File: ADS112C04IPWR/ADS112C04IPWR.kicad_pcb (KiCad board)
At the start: 2 copper layers, 22.9 x 22.9 mm, 3 parts, among them J1 Conn_01x08, J2 Conn_01x08, U1 ADS112C04IPWR

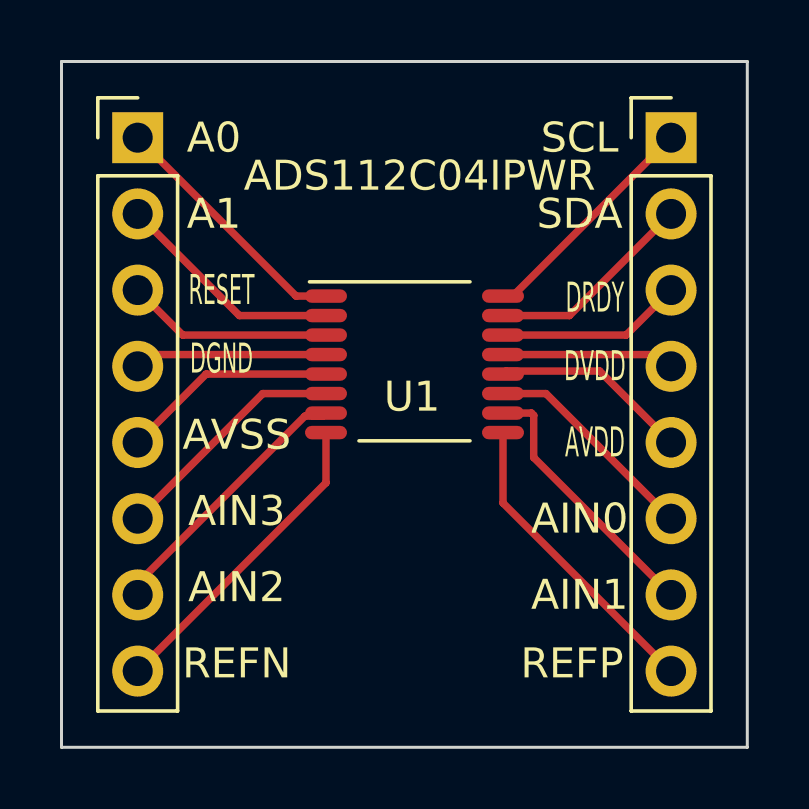
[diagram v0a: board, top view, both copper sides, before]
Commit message: Revision One
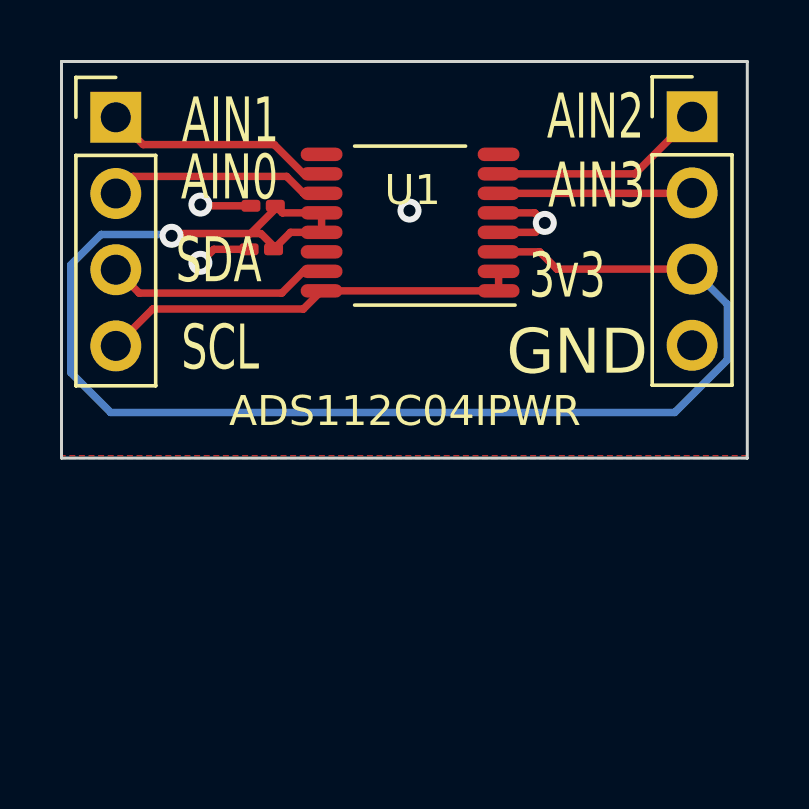
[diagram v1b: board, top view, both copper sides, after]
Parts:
- added C1: 0.1μF, Capacitor_SMD:C_0201_0603Metric_Pad0.64x0.40mm_HandSolder, F.Cu at (149.0, 68.3)
- added C2: 0.1μF, Capacitor_SMD:C_0201_0603Metric_Pad0.64x0.40mm_HandSolder, F.Cu at (148.9, 69.8)
- J1, J2: value Conn_01x08 -> Conn_01x04; footprint Connector_PinHeader_2.54mm:PinHeader_1x08_P2.54mm_Vertical -> Connector_PinHeader_2.54mm:PinHeader_1x04_P2.54mm_Vertical
- moved U1 4.73 mm to (153.9, 68.9), turned to 180 degrees
- moved J1 1.00 mm to (144.1, 65.4)
- moved J2 0.99 mm to (163.3, 65.3)
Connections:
- J1 pad 1: Net-(J1-Pad1) -> /AIN1
- J1 pad 2: Net-(J1-Pad2) -> /AIN0
- J1 pad 3: Net-(J1-Pad3) -> /SDA
- J1 pad 4: GNDD -> /SCL
- J2 pad 1: Net-(J2-Pad1) -> /AIN2
- J2 pad 2: Net-(J2-Pad2) -> /AIN3
- J2 pad 3: Net-(J2-Pad3) -> +3V3
- J2 pad 4: Net-(J2-Pad4) -> GND
- U1 pad 1: Net-(J1-Pad1) -> /SCL
- U1 pad 10: Net-(J2-Pad7) -> /AIN1
- U1 pad 11: Net-(J2-Pad6) -> /AIN0
- U1 pad 12: Net-(J2-Pad5) -> +3V3
- U1 pad 13: Net-(J2-Pad4) -> +3V3
- U1 pad 14: Net-(J2-Pad3) -> unconnected-(U1-Pad14)
- U1 pad 15: Net-(J2-Pad2) -> /SDA
- U1 pad 16: Net-(J2-Pad1) -> /SCL
- U1 pad 2: Net-(J1-Pad2) -> /SCL
- U1 pad 3: Net-(J1-Pad3) -> +3V3
- U1 pad 4: GNDD -> GND
- U1 pad 5: Net-(J1-Pad5) -> GND
- U1 pad 6: Net-(J1-Pad6) -> /AIN3
- U1 pad 7: Net-(J1-Pad7) -> /AIN2
- U1 pad 8: Net-(J1-Pad8) -> unconnected-(U1-Pad8)
- U1 pad 9: Net-(J2-Pad8) -> unconnected-(U1-Pad9)
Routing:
- net +3V3: track 0.00 -> 49.9 mm, vias 0 -> 1
- net /SCL: track 0.00 -> 14.2 mm
- net Net-(J1-Pad8): track 10.6 -> 0.00 mm
- net Net-(J2-Pad8): track 10.3 -> 0.00 mm
- net Net-(J1-Pad7): track 9.01 -> 0.00 mm
- net Net-(J2-Pad7): track 8.94 -> 0.00 mm
- net Net-(J1-Pad1): track 8.46 -> 0.00 mm
- net Net-(J1-Pad6): track 8.00 -> 0.00 mm
- net Net-(J2-Pad1): track 7.79 -> 0.00 mm
- net Net-(J1-Pad2): track 7.68 -> 0.00 mm
- net /AIN1: track 0.00 -> 7.64 mm
- net /SDA: track 0.00 -> 7.48 mm
- net Net-(J2-Pad6): track 7.33 -> 0.00 mm
- net /AIN0: track 0.00 -> 7.33 mm
- net /AIN2: track 0.00 -> 7.24 mm
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- added copper zone on B.Cu, net GND
- added copper zone on F.Cu, net GND
- removed copper zone on B.Cu, net GNDD
- removed copper zone on F.Cu, net GNDD
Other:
- board size 22.9 x 22.9 mm -> 22.9 x 13.2 mm
- board text added: "3v3"
- board text added: "GND"
- board text added: "I²C address 100 1111 (0x4F)"
- board text removed: "A0"
- board text removed: "A1"
- board text removed: "AVDD"
- board text removed: "AVSS"
- board text removed: "DGND"
- board text removed: "DRDY"
- board text removed: "DVDD"
- board text removed: "REFN"
- board text removed: "REFP"
- board text removed: "RESET"
